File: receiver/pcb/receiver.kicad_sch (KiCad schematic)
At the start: 22 parts, among them M1 Conn_01x02_Female, M2 Conn_01x02_Female, U1 DRV8870DDA, U2 DRV8870DDA

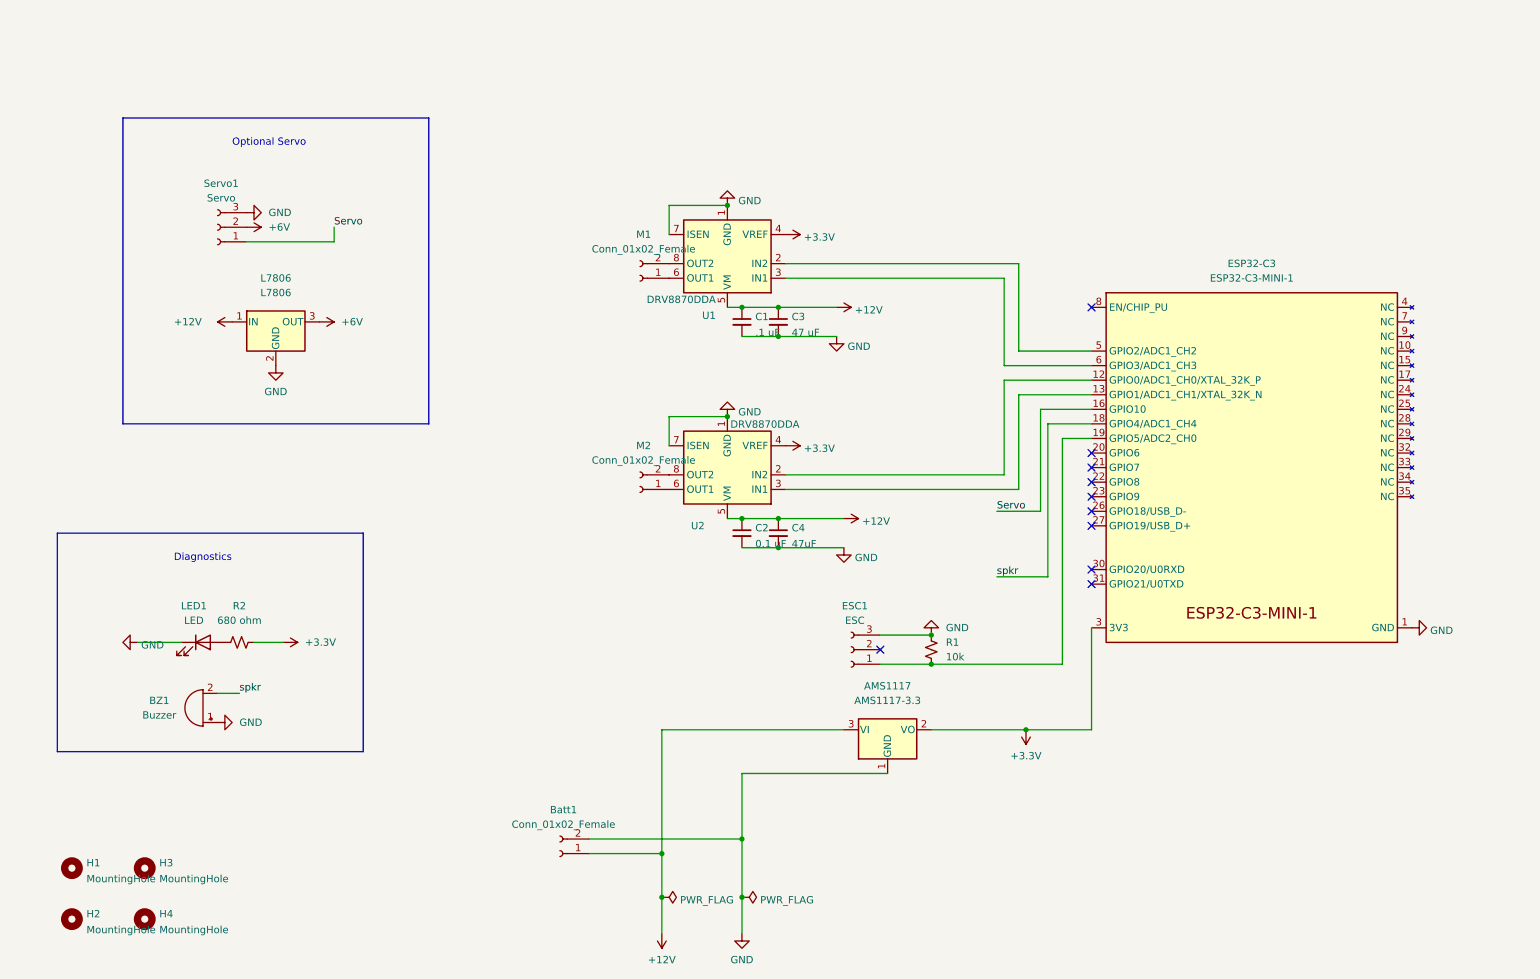
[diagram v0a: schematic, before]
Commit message: receiver V4 ordered
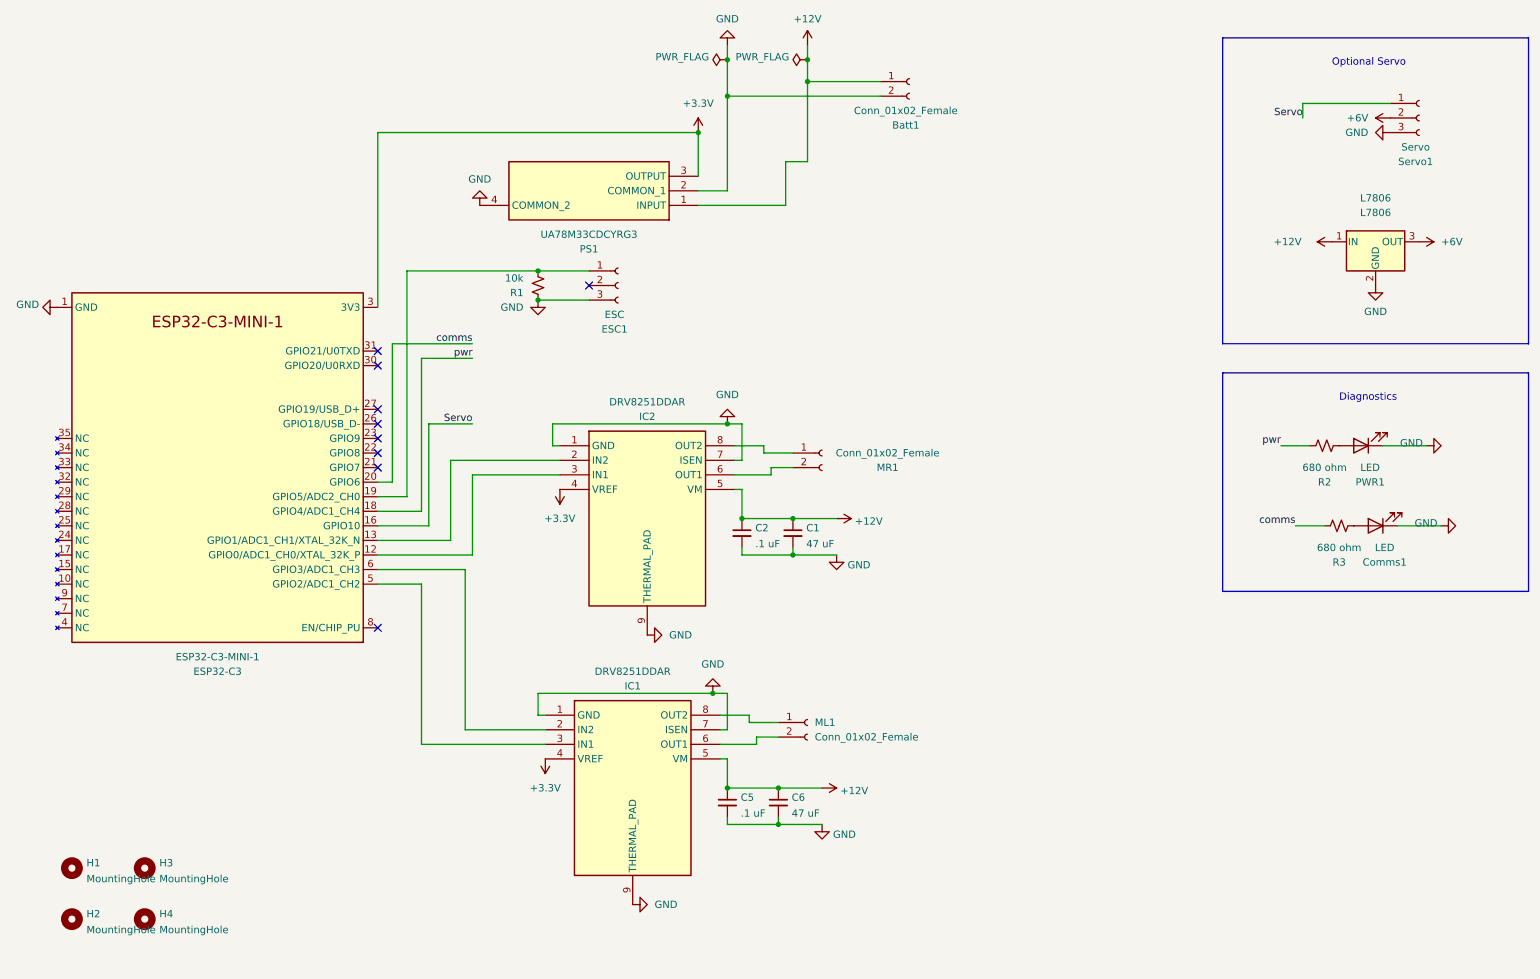
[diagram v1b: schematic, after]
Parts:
- removed AMS1117: AMS1117-3.3, Package_TO_SOT_SMD:SOT-223-3_TabPin2, symbol Regulator_Linear:AMS1117-3.3
- removed BZ1: Buzzer, Buzzer_Beeper:Buzzer_CUI_CPT-9019S-SMT, symbol Device:Buzzer
- removed C3: 47 uF, Capacitor_SMD:C_0805_2012Metric_Pad1.18x1.45mm_HandSolder, symbol Device:C_Small
- removed C4: 47uF, Capacitor_SMD:C_0805_2012Metric_Pad1.18x1.45mm_HandSolder, symbol Device:C_Small
- removed M1, M2: Conn_01x02_Female, Connector_PinSocket_2.54mm:PinSocket_1x02_P2.54mm_Vertical, symbol Connector:Conn_01x02_Female
- removed U1, U2: DRV8870DDA, Package_SO:Texas_HTSOP-8-1EP_3.9x4.9mm_P1.27mm_EP2.95x4.9mm_Mask2.4x3.1mm_ThermalVias, symbol Driver_Motor:DRV8870DDA
- added C5: .1 uF, Capacitor_SMD:C_0805_2012Metric_Pad1.18x1.45mm_HandSolder, symbol Device:C_Small
- added C6: 47 uF, Capacitor_SMD:C_0805_2012Metric_Pad1.18x1.45mm_HandSolder, symbol Device:C_Small
- added Comms1: LED, LED_SMD:LED_0805_2012Metric_Pad1.15x1.40mm_HandSolder, symbol Device:LED
- added IC1, IC2: DRV8251DDAR, drv8251:SOIC127P600X170-9N, symbol DRV8251:DRV8251DDAR
- added ML1, MR1: Conn_01x02_Female, Connector_PinSocket_2.54mm:PinSocket_1x02_P2.54mm_Vertical, symbol Connector:Conn_01x02_Female
- added PS1: UA78M33CDCYRG3, ua78-vreg:SOT230P700X180-4N, symbol libraries:UA78M33CDCYRG3
- added R3: 680 ohm, Resistor_SMD:R_0805_2012Metric_Pad1.20x1.40mm_HandSolder, symbol Device:R_Small_US
- C1: value .1 uF -> 47 uF
- C2: value 0.1 uF -> .1 uF
- renumbered LED1 to PWR1
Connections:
- net +12V: now also C5.1, C6.1, IC1.5 (VM), IC2.5 (VM), PS1.1 (INPUT)
- net +3V3: now also IC1.4 (VREF), IC2.4 (VREF), PS1.3 (OUTPUT); no longer R2.1
- net GND: now also C5.2, C6.2, Comms1.1 (K), IC1.1 (GND), IC1.7 (ISEN), IC1.9 (THERMAL_PAD), IC2.1 (GND), IC2.7 (ISEN), IC2.9 (THERMAL_PAD), PS1.2 (COMMON_1), PS1.4 (COMMON_2)
- net at ESP32-C3.12 (GPIO0/ADC1_CH0/XTAL_32K_P): now also IC2.3 (IN1)
- net at ESP32-C3.13 (GPIO1/ADC1_CH1/XTAL_32K_N): now also IC2.2 (IN2)
- net comms: now reaches ESP32-C3.20 (GPIO6)
- net comms: now also R3.1
- net at ESP32-C3.5 (GPIO2/ADC1_CH2): now also IC1.3 (IN1)
- net at ESP32-C3.6 (GPIO3/ADC1_CH3): now also IC1.2 (IN2)
- net spkr renamed pwr
- net pwr: now also R2.1
- new net: Comms1.2 (A), R3.2
- new net: IC1.8 (OUT2), ML1.1 (Pin_1)
- new net: IC1.6 (OUT1), ML1.2 (Pin_2)
- new net: IC2.6 (OUT1), MR1.2 (Pin_2)
- new net: IC2.8 (OUT2), MR1.1 (Pin_1)
- no-connect marks 10 -> 9
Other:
- moved on the sheet: Batt1, ESC1, ESP32-C3, L7806, PWR1, R1, R2, Servo1
